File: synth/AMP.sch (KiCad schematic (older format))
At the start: 17 parts, among them J2 Screw_Terminal_01x02, Q3 Q_NMOS_SGD, Q4 Q_PMOS_SGD, SW3 SW_SPDT, U4 MCP6002

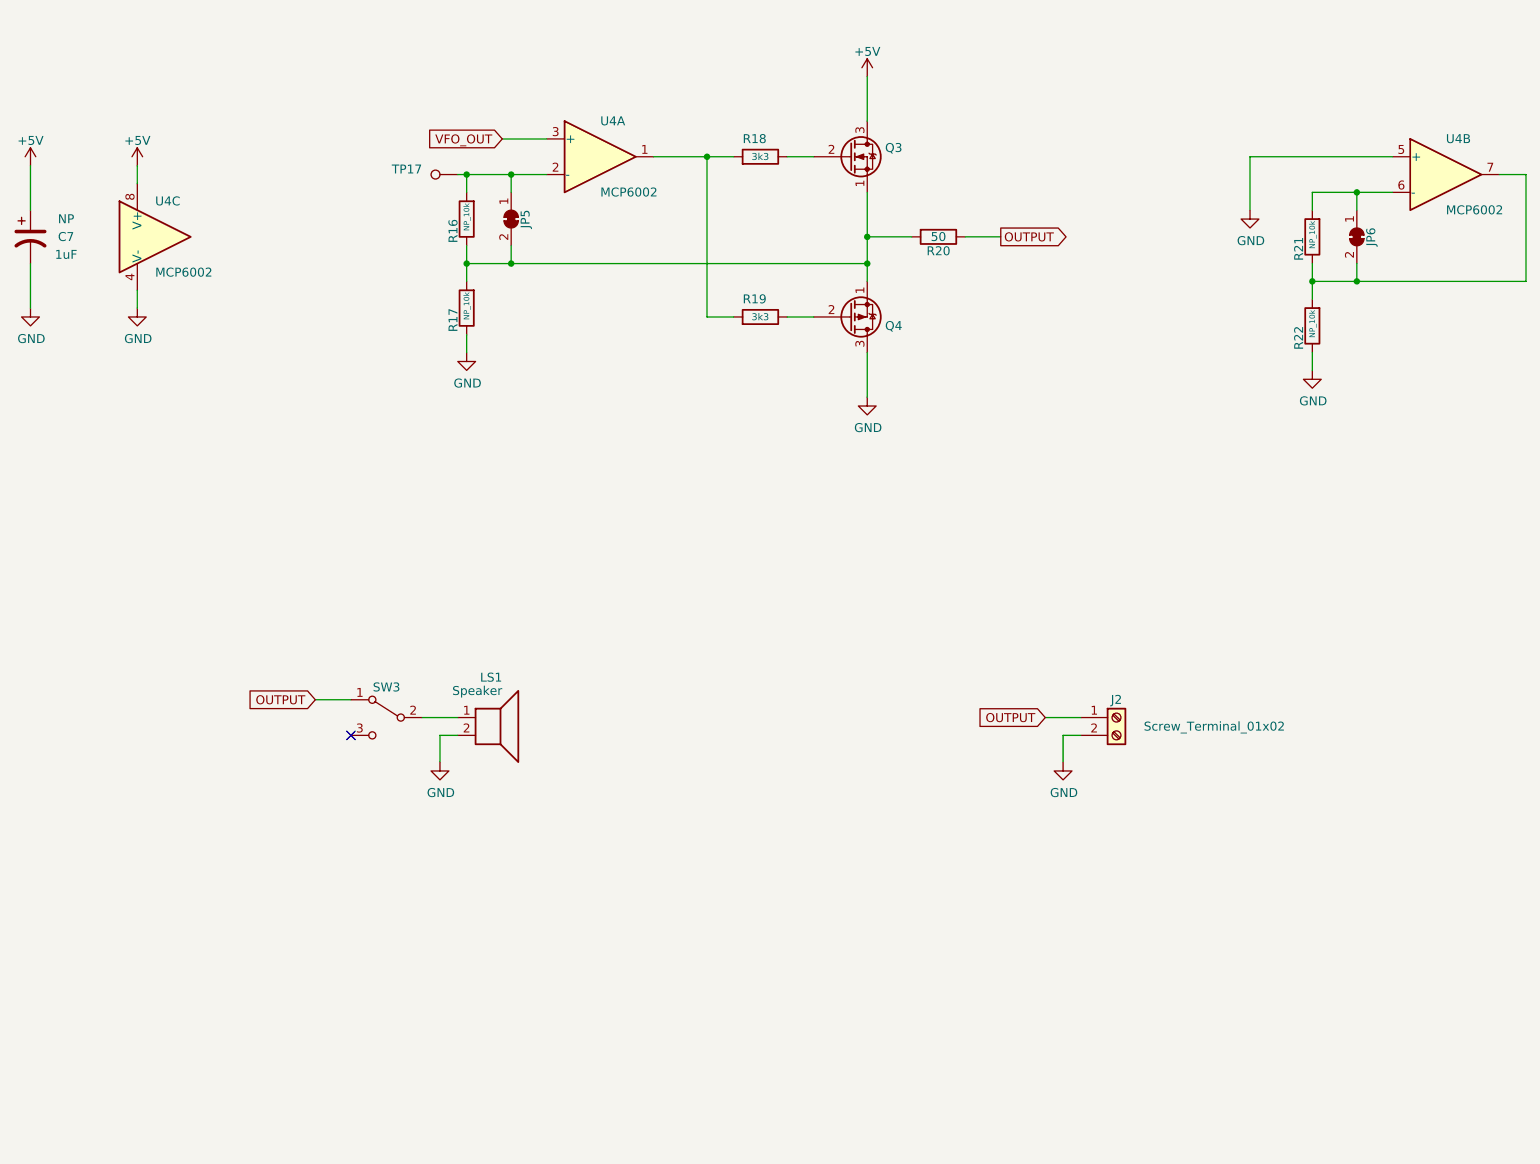
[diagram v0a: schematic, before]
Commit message: automated commit
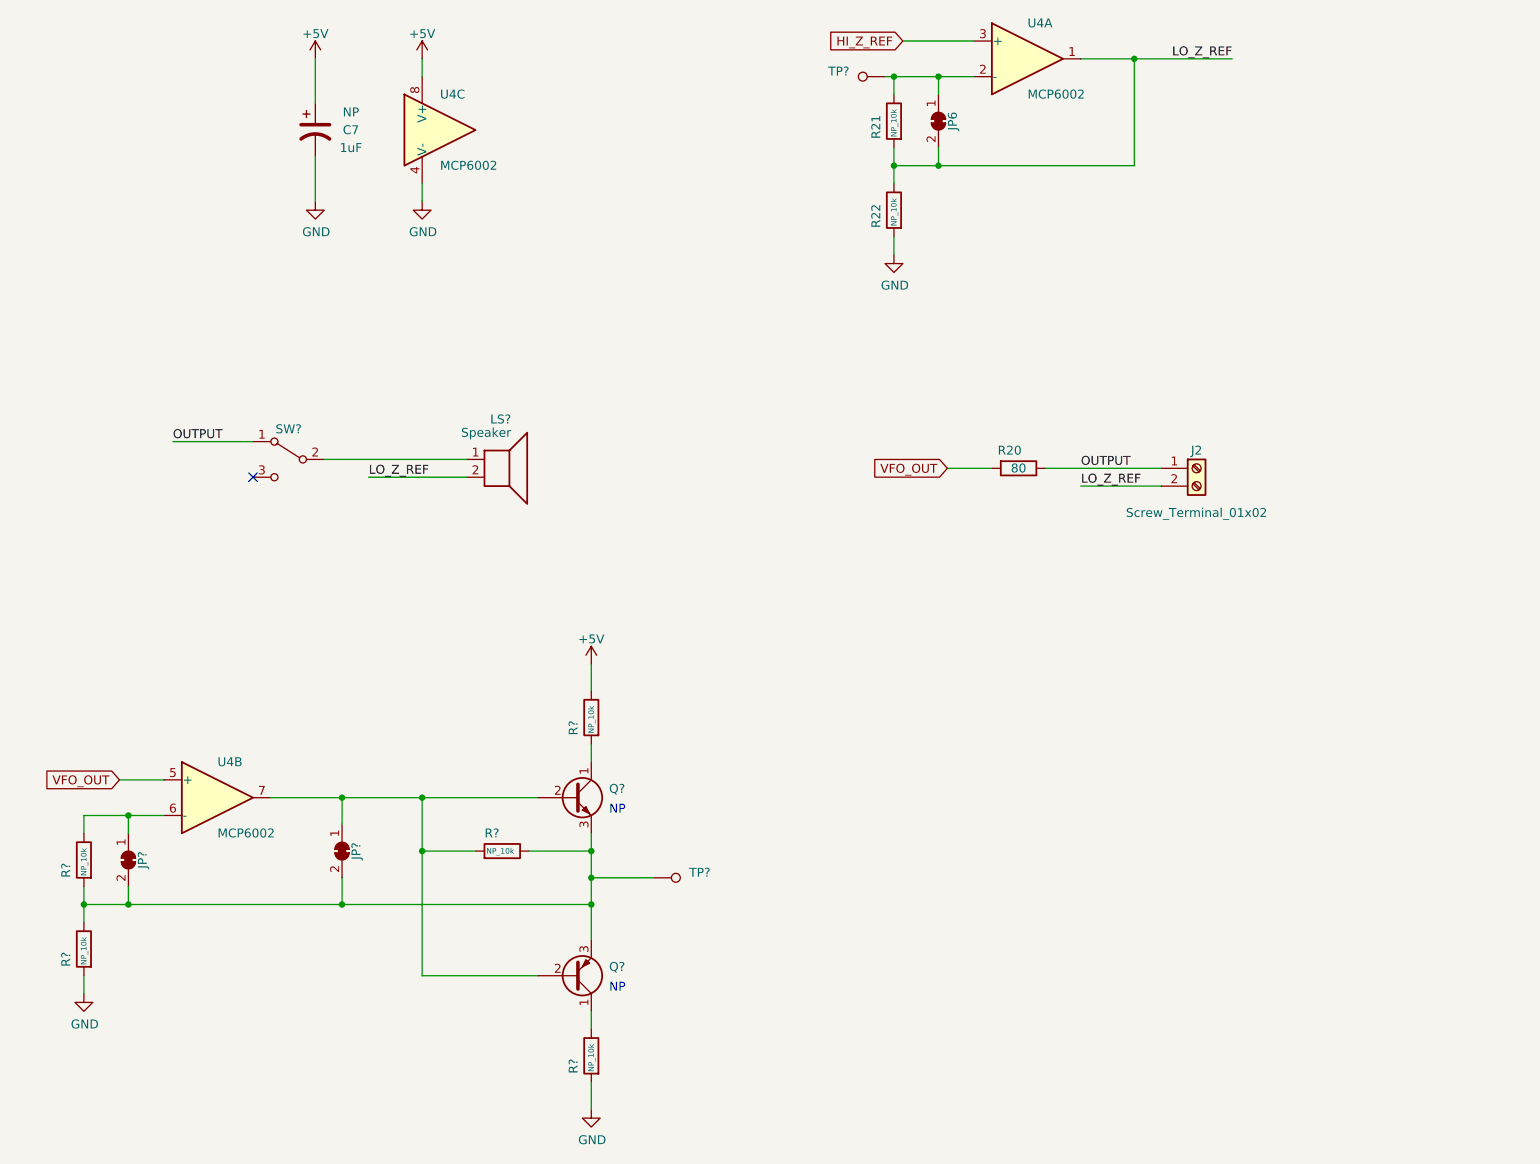
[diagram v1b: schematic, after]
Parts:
- removed JP5: SolderJumper_2_Bridged, symbol Jumper:SolderJumper_2_Bridged
- removed LS1: Speaker, symbol Device:Speaker
- removed Q3: Q_NMOS_SGD, symbol Device:Q_NMOS_SGD
- removed Q4: Q_PMOS_SGD, symbol Device:Q_PMOS_SGD
- removed R16, R17: NP_10k, symbol Device:R
- removed R18, R19: 3k3, symbol Device:R
- removed SW3: SW_SPDT, symbol Switch:SW_SPDT
- removed TP17: PTH_1_mm, TestPoint:TestPoint_THTPad_D2.0mm_Drill1.0mm, symbol custom:PTH_1_mm
- added JP? (x2): SolderJumper_2_Bridged, symbol Jumper:SolderJumper_2_Bridged
- added LS?: Speaker, symbol Device:Speaker
- added Q?: Q_PNP_CBE, symbol Device:Q_PNP_CBE
- added Q?: Q_NPN_CBE, symbol Device:Q_NPN_CBE
- added R? (x5): NP_10k, symbol Device:R
- added SW?: SW_SPDT, symbol Switch:SW_SPDT
- added TP? (x2): PTH_1_mm, TestPoint:TestPoint_THTPad_D2.0mm_Drill1.0mm, symbol custom:PTH_1_mm
- R20: value 50 -> 80
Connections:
- net +5V: now also R?.1
- net GND: now also R22.2, R?.2, R?.2; no longer J2.2 (Pin_2), R22.1, U4.5 (+)
- net OUTPUT: now also SW?.1 (A)
- net VFO_OUT: now also R20.2, U4.5 (+); no longer U4.3 (+)
- net LO_Z_REF: now reaches U4.1
- net LO_Z_REF: now also J2.2 (Pin_2), JP6.2 (B), R21.2, R22.1, LS?.2
- net at U4.2 (-): now also JP6.1 (A), R21.1, TP?.1
- new net: Q?.1 (C), R?.1
- new net: JP?.1 (A), Q?.2 (B), Q?.2 (B), R?.2, U4.7
- new net: JP?.2 (B), JP?.2 (B), Q?.3 (E), Q?.3 (E), R?.1, R?.1, R?.2, TP?.1
- new net: Q?.1 (C), R?.2
- new net: JP?.1 (A), R?.1, U4.6 (-)
- new net: LS?.1, SW?.2 (B)
- new net HI_Z_REF: U4.3 (+)
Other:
- note added: "NP"
- moved on the sheet: C7, J2, JP6, R20, R21, R22, U4A, U4B, U4C
